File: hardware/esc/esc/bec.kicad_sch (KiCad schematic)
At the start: 10 parts, among them IC2 LM5148QRGYRQ1, Q1 NX138AKHH, Q3 BUK9K12-80LX

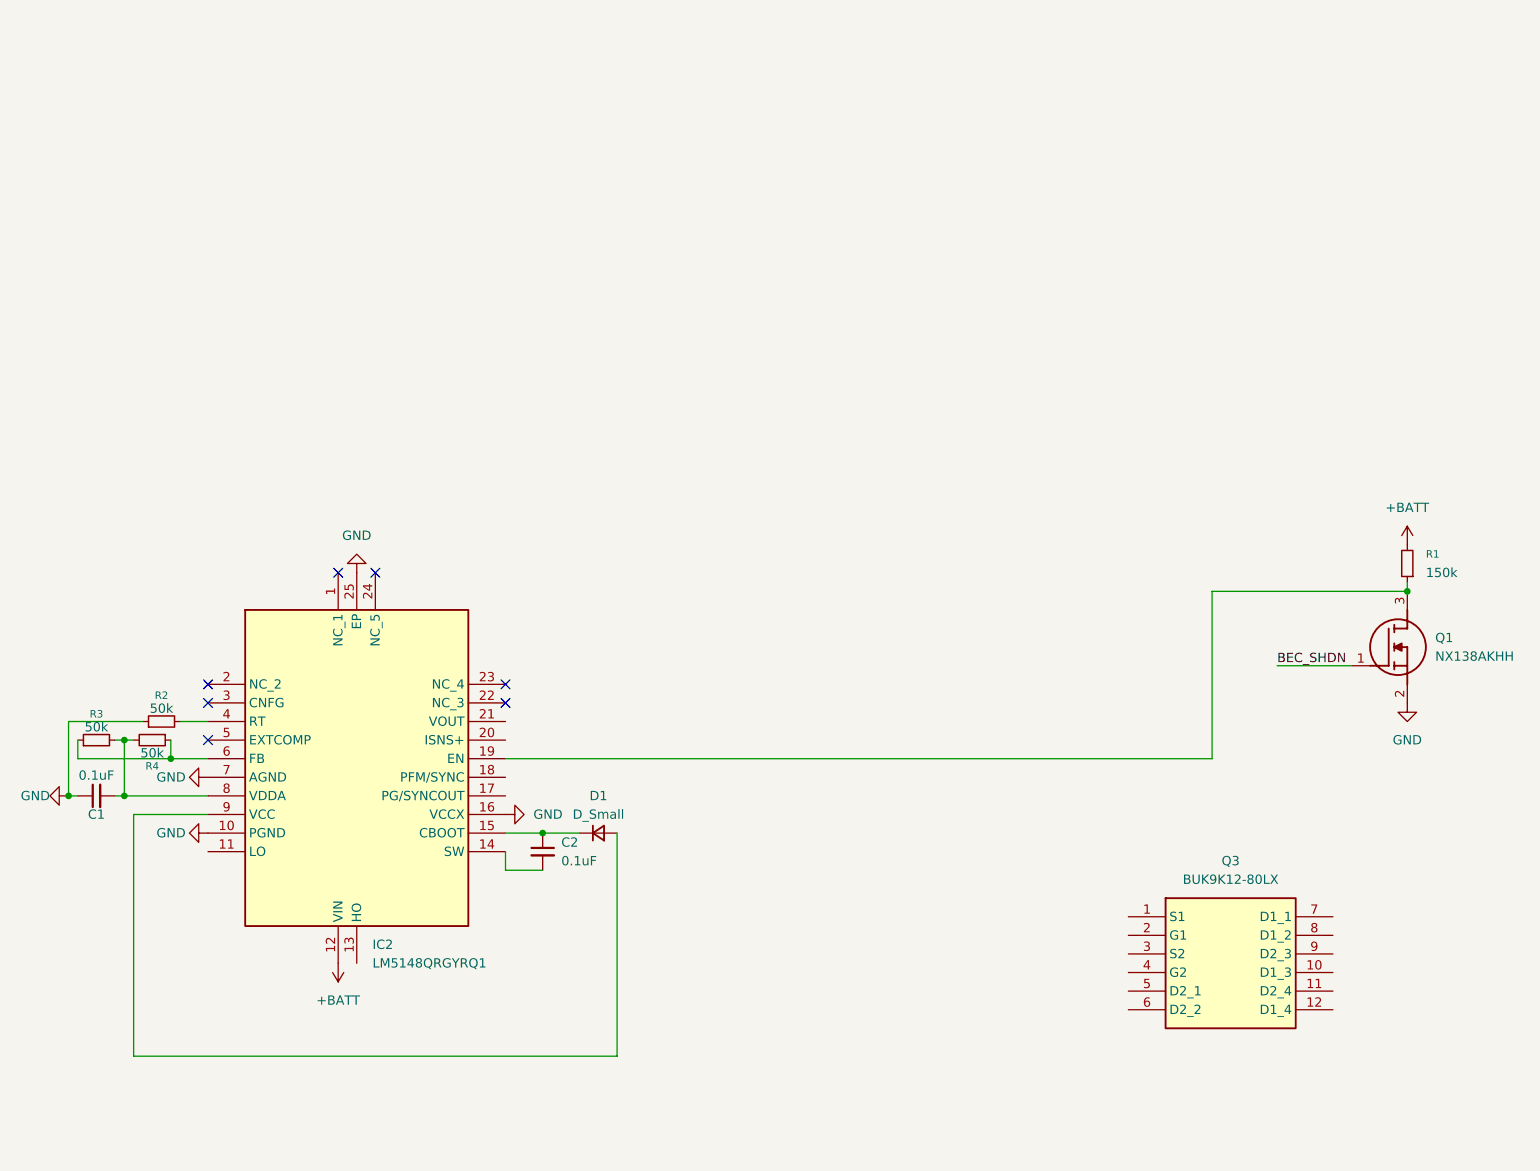
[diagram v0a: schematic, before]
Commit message: more pcb stuff
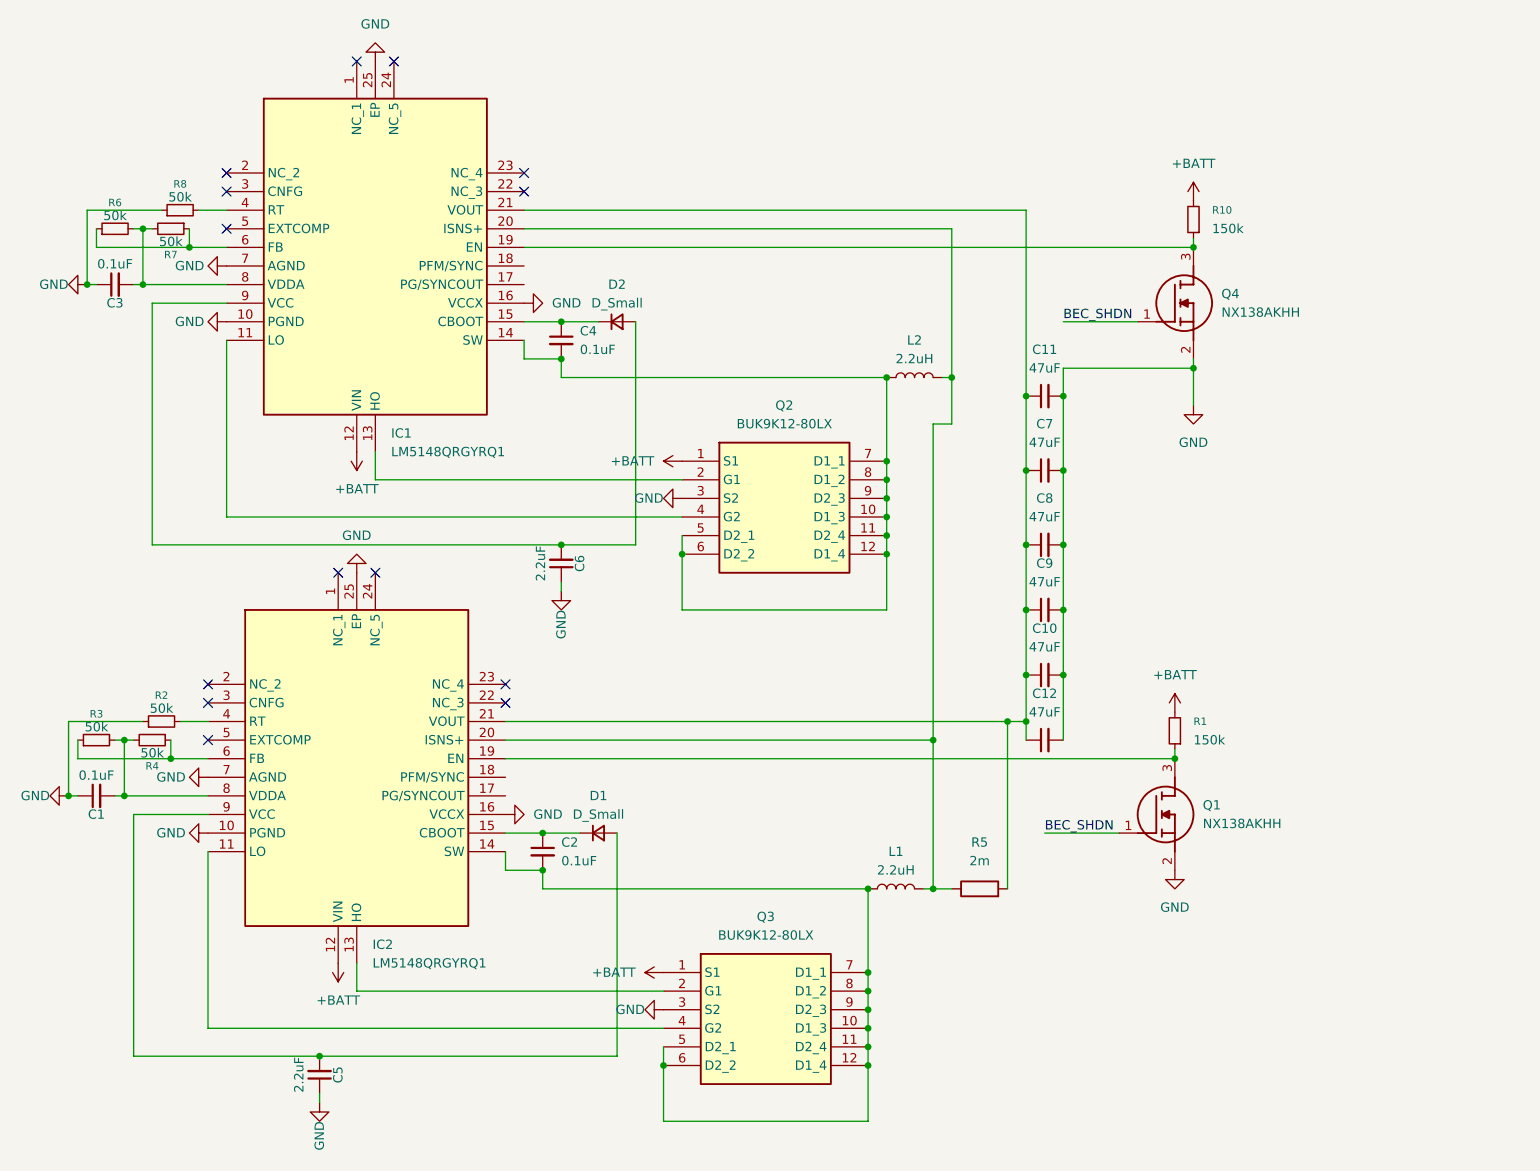
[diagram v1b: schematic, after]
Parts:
- added C10, C11, C12, C7, C8, C9: 47uF, symbol Device:C_Small
- added C3, C4: 0.1uF, Capacitor_SMD:C_0603_1608Metric, symbol Device:C_Small
- added C5, C6: 2.2uF, Capacitor_SMD:C_0603_1608Metric, symbol Device:C_Small
- added D2: D_Small, Diode_SMD:D_0603_1608Metric_Pad1.05x0.95mm_HandSolder, symbol Device:D_Small
- added IC1: LM5148QRGYRQ1, LM5148QRGYRQ1, symbol LM5148QRGYRQ1:LM5148QRGYRQ1
- added L1, L2: 2.2uH, Inductor_SMD:L_APV_APH1770, symbol Device:L
- added Q2: BUK9K12-80LX, BUK7K6R840E115, symbol BUK9K12-80LX:BUK9K12-80LX
- added Q4: NX138AKHH, NX138AKHH, symbol NX138AKHH:NX138AKHH
- added R10: 150k, symbol Device:R_Small
- added R5: 2m, Resistor_SMD:R_2512_6332Metric, symbol Device:R
- added R6, R7, R8: 50k, Resistor_SMD:R_0402_1005Metric, symbol Device:R_Small
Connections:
- net +BATT: now also Q3.1 (S1), IC1.12 (VIN), Q2.1 (S1), R10.2
- net BEC_SHDN: now also Q4.1 (G)
- net GND: now also Q3.3 (S2), C10.2, C11.2, C12.2, C3.1, C5.1, C6.1, C7.2, C8.2, C9.2, IC1.10 (PGND), IC1.16 (VCCX), IC1.25 (EP), IC1.7 (AGND), Q2.3 (S2), Q4.2 (S), R8.1
- net at IC2.11 (LO): now also Q3.4 (G2)
- net at IC2.13 (HO): now also Q3.2 (G1)
- net at C2.2, IC2.14 (SW): now also Q3.10 (D1_3), Q3.11 (D2_4), Q3.12 (D1_4), Q3.5 (D2_1), Q3.6 (D2_2), Q3.7 (D1_1), Q3.8 (D1_2), Q3.9 (D2_3), L1.1
- net at IC2.20 (ISNS+): now also IC1.20 (ISNS+), L1.2, L2.2, R5.1
- net at IC2.21 (VOUT): now also C10.1, C11.1, C12.1, C7.1, C8.1, C9.1, IC1.21 (VOUT), R5.2
- net at D1.2 (A), IC2.9 (VCC): now also C5.2
- new net: C4.1, D2.1 (K), IC1.15 (CBOOT)
- new net: C4.2, IC1.14 (SW), L2.1, Q2.10 (D1_3), Q2.11 (D2_4), Q2.12 (D1_4), Q2.5 (D2_1), Q2.6 (D2_2), Q2.7 (D1_1), Q2.8 (D1_2), Q2.9 (D2_3)
- new net: C6.2, D2.2 (A), IC1.9 (VCC)
- new net: IC1.6 (FB), R6.1, R7.1
- new net: C3.2, IC1.8 (VDDA), R6.2, R7.2
- new net: IC1.4 (RT), R8.2
- new net: IC1.19 (EN), Q4.3 (D), R10.1
- new net: IC1.11 (LO), Q2.4 (G2)
- new net: IC1.13 (HO), Q2.2 (G1)
- no-connect marks 7 -> 14
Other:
- moved on the sheet: Q1, Q3, R1
